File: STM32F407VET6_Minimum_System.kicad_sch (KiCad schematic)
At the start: 20 parts, among them SW1 SW_DIP_x01, U1 STM32F407VET, Y1 8MHz

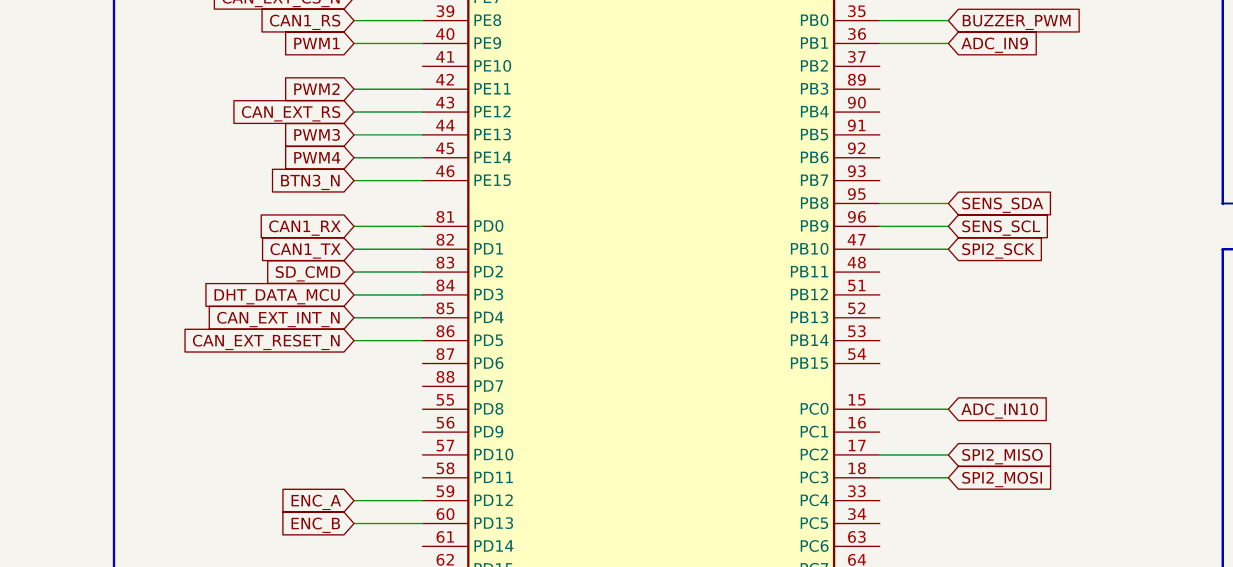
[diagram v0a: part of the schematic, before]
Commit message: feat: implement precision adc
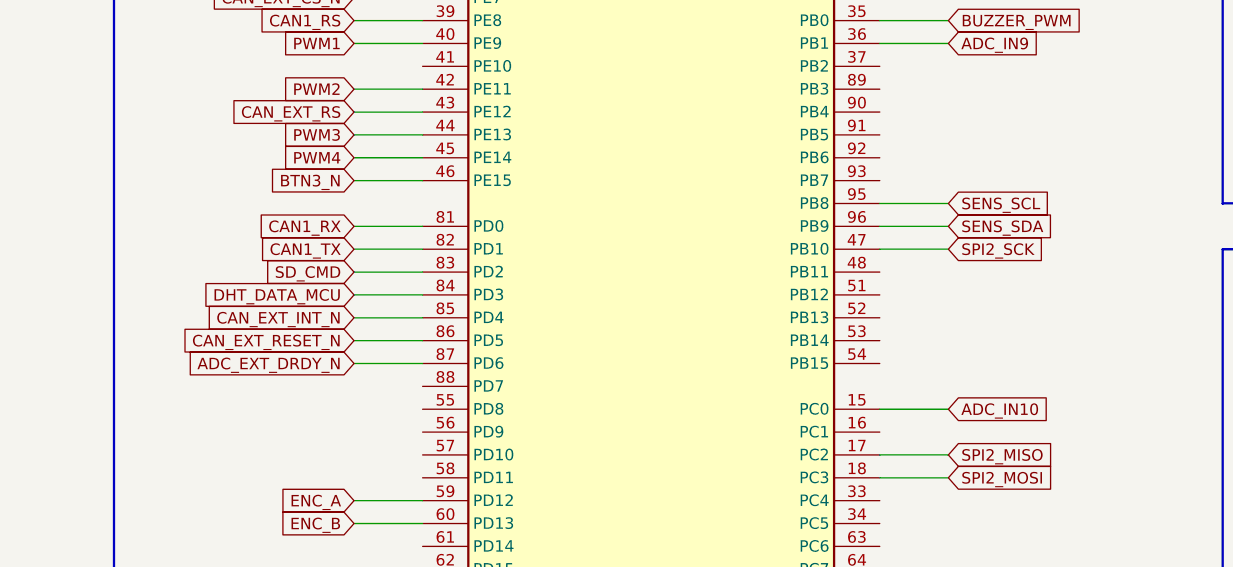
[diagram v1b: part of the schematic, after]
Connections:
- net SENS_SCL: now also U1.95 (PB8); no longer U1.96 (PB9)
- net SENS_SDA: now also U1.96 (PB9); no longer U1.95 (PB8)
- net ADC_EXT_DRDY_N: now reaches U1.87 (PD6)
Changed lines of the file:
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@@
+	(wire
+		(pts
+			(xy 172.72 132.08) (xy 180.34 132.08)
+		)
+		(stroke
+			(width 0)
+			(type default)
+		)
+	)
 	(wire
 		(pts
@@
 				)
 				(justify left)
+			)
+		)
+	)
+	(global_label "ADC_EXT_DRDY_N"
+		(shape input)
+		(at 172.72 132.08 180)
+		(fields_autoplaced yes)
+		(effects
+			(font
+				(size 1.27 1.27)
+			)
+			(justify right)
+		)
+		(property "Intersheetrefs" "${INTERSHEET_REFS}"
+			(at 153.6482 132.08 0)
+			(hide yes)
+			(show_name no)
+			(do_not_autoplace no)
+			(effects
+				(font
+					(size 1.27 1.27)
+				)
+				(justify right)
 			)
 		)
@@
 	(global_label "SENS_SCL"
 		(shape input)
-		(at 238.76 116.84 0)
+		(at 238.76 114.3 0)
 		(fields_autoplaced yes)
 		(effects
@@
 		)
 		(property "Intersheetrefs" "${INTERSHEET_REFS}"
-			(at 251.1189 116.84 0)
+			(at 251.1189 114.3 0)
 			(hide yes)
 			(show_name no)
@@
 	(global_label "SENS_SDA"
 		(shape input)
-		(at 238.76 114.3 0)
+		(at 238.76 116.84 0)
 		(fields_autoplaced yes)
 		(effects
@@
 		)
 		(property "Intersheetrefs" "${INTERSHEET_REFS}"
-			(at 251.1794 114.3 0)
-			(hide yes)
-			(show_name no)
+			(at 251.1794 116.84 0)
+			(hide yes)
+			(show_name no)
